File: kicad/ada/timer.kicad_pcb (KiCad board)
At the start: 2 copper layers, 70 x 100 mm, 27 parts, among them IC1 ATMEGA328P-A, P1 BATTERY, P2 ICSP, Q1 NMOS, Q2 PMOS, SW1 SPST, U1 TOUCH_PAD_13, U2 MTCH6102_SSOP, U3 MCP1755ST-3302E/DB, U4 APA_102C

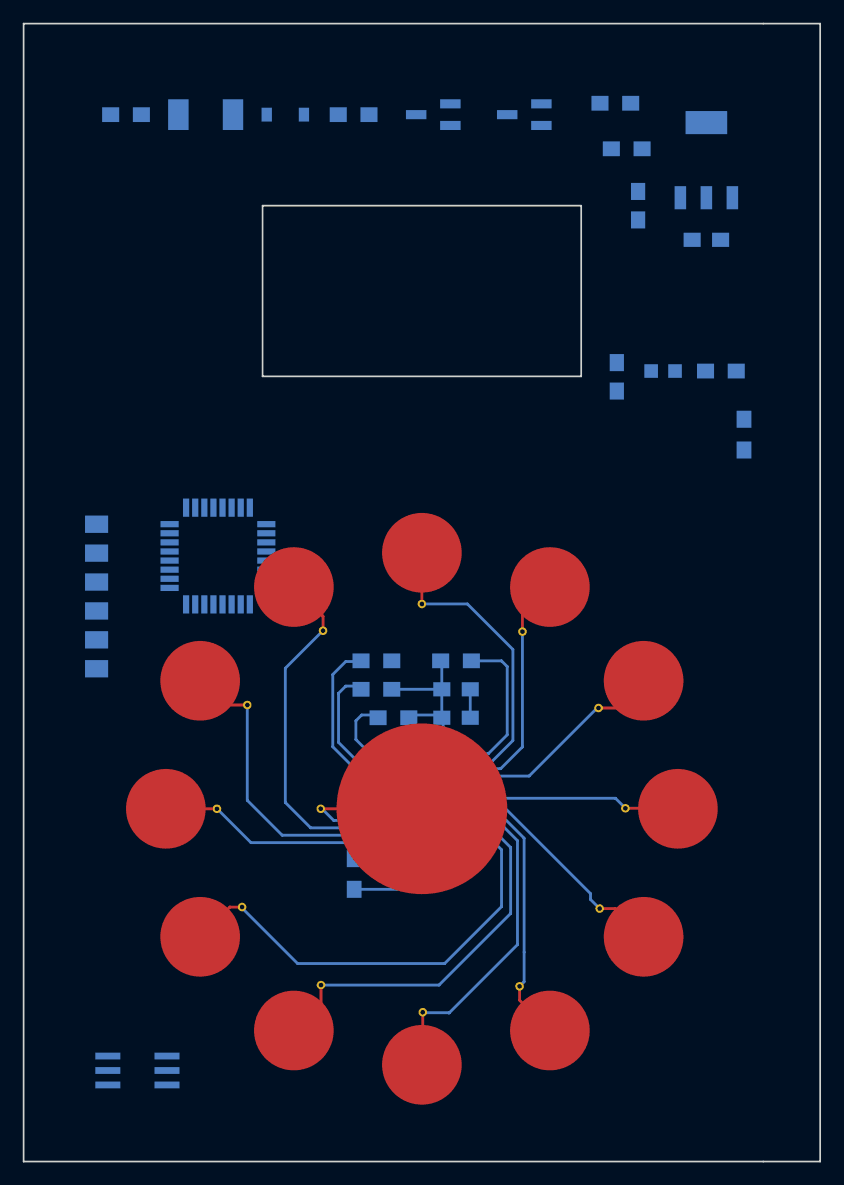
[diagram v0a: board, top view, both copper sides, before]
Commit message: Start of using clockface
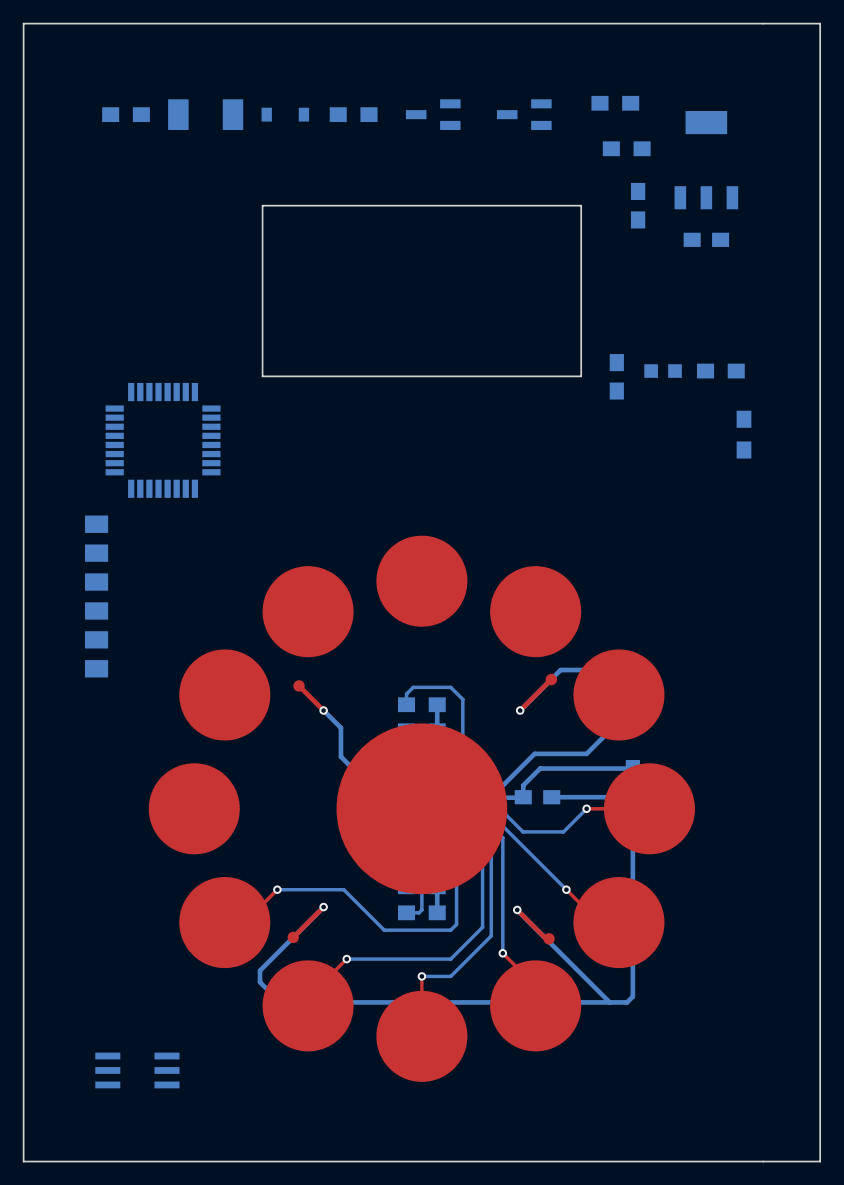
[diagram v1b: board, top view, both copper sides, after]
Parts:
- removed R5: 4.7k, Resistors_SMD:R_0805_HandSoldering
- P2: footprint SIP-6-SMD -> touch_timer:SIP-6-SMD
- U1: footprint touch_circle -> touch_timer:CPA_12
- U2: footprint Housings_SSOP:SSOP-28_5.3x10.2mm_Pitch0.65mm -> touch_timer:SSOP-28_5.3x10.2mm_Pitch0.65mm_masked
- moved R4 22.5 mm to (150.0, 113.1)
- moved C2 17.6 mm to (168.5, 101.7), turned to 270 degrees
- moved IC1 11.2 mm to (127.3, 71.6)
- moved C1 10.0 mm to (160.2, 103.0)
- moved R1 6.06 mm to (150.0, 110.9), turned to 180 degrees
- moved R3 4.89 mm to (150.0, 94.9), turned to 180 degrees
- moved R2 2.75 mm to (150.0, 97.1)
- moved U2 0.85 mm to (150.0, 104.0)
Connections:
- net VCC renamed /VCC
- U2 pad 12: /SYNC -> Net-(U2-Pad12)
- U4 pad 4: /POWER -> /3V3
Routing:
- net GND: track 2.50 -> 131.1 mm, vias 0 -> 4
- net /RX11: track 31.3 -> 1.28 mm
- net /RX0: track 26.8 -> 0.07 mm
- net /RX10: track 27.2 -> 2.01 mm
- net /RX1: track 24.0 -> 1.50 mm
- net /RX9: track 20.7 -> 0.00 mm
- net /RX2: track 22.2 -> 1.57 mm
- net /RX12: track 15.0 -> 0.00 mm
- net /SYNC: track 11.9 -> 0.00 mm
- net /RX8: track 40.1 -> 32.4 mm, vias 0 -> 1
- net /RX4: track 23.9 -> 17.7 mm, vias 0 -> 1
- net /RX6: track 29.7 -> 24.6 mm, vias 0 -> 1
- net /RX7: track 34.6 -> 29.9 mm, vias 0 -> 1
- net /RX5: track 23.9 -> 20.1 mm, vias 0 -> 1
- net /SDA: track 7.26 -> 4.58 mm
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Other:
- net class Default: trace_width 0.25 -> 0.305
- net class GND added: clearance 0.2, trace_width 0.406, via_dia 0.75, via_drill 0.4
- net class VCC added: clearance 0.2, trace_width 0.406, via_dia 0.75, via_drill 0.4
